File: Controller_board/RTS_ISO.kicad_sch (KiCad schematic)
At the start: 18 parts, among them U7 ADuM1400xRW SOIC-16W, U8 ADuM1400xRW SOIC-16W, U9 ADuM1400xRW SOIC-16W

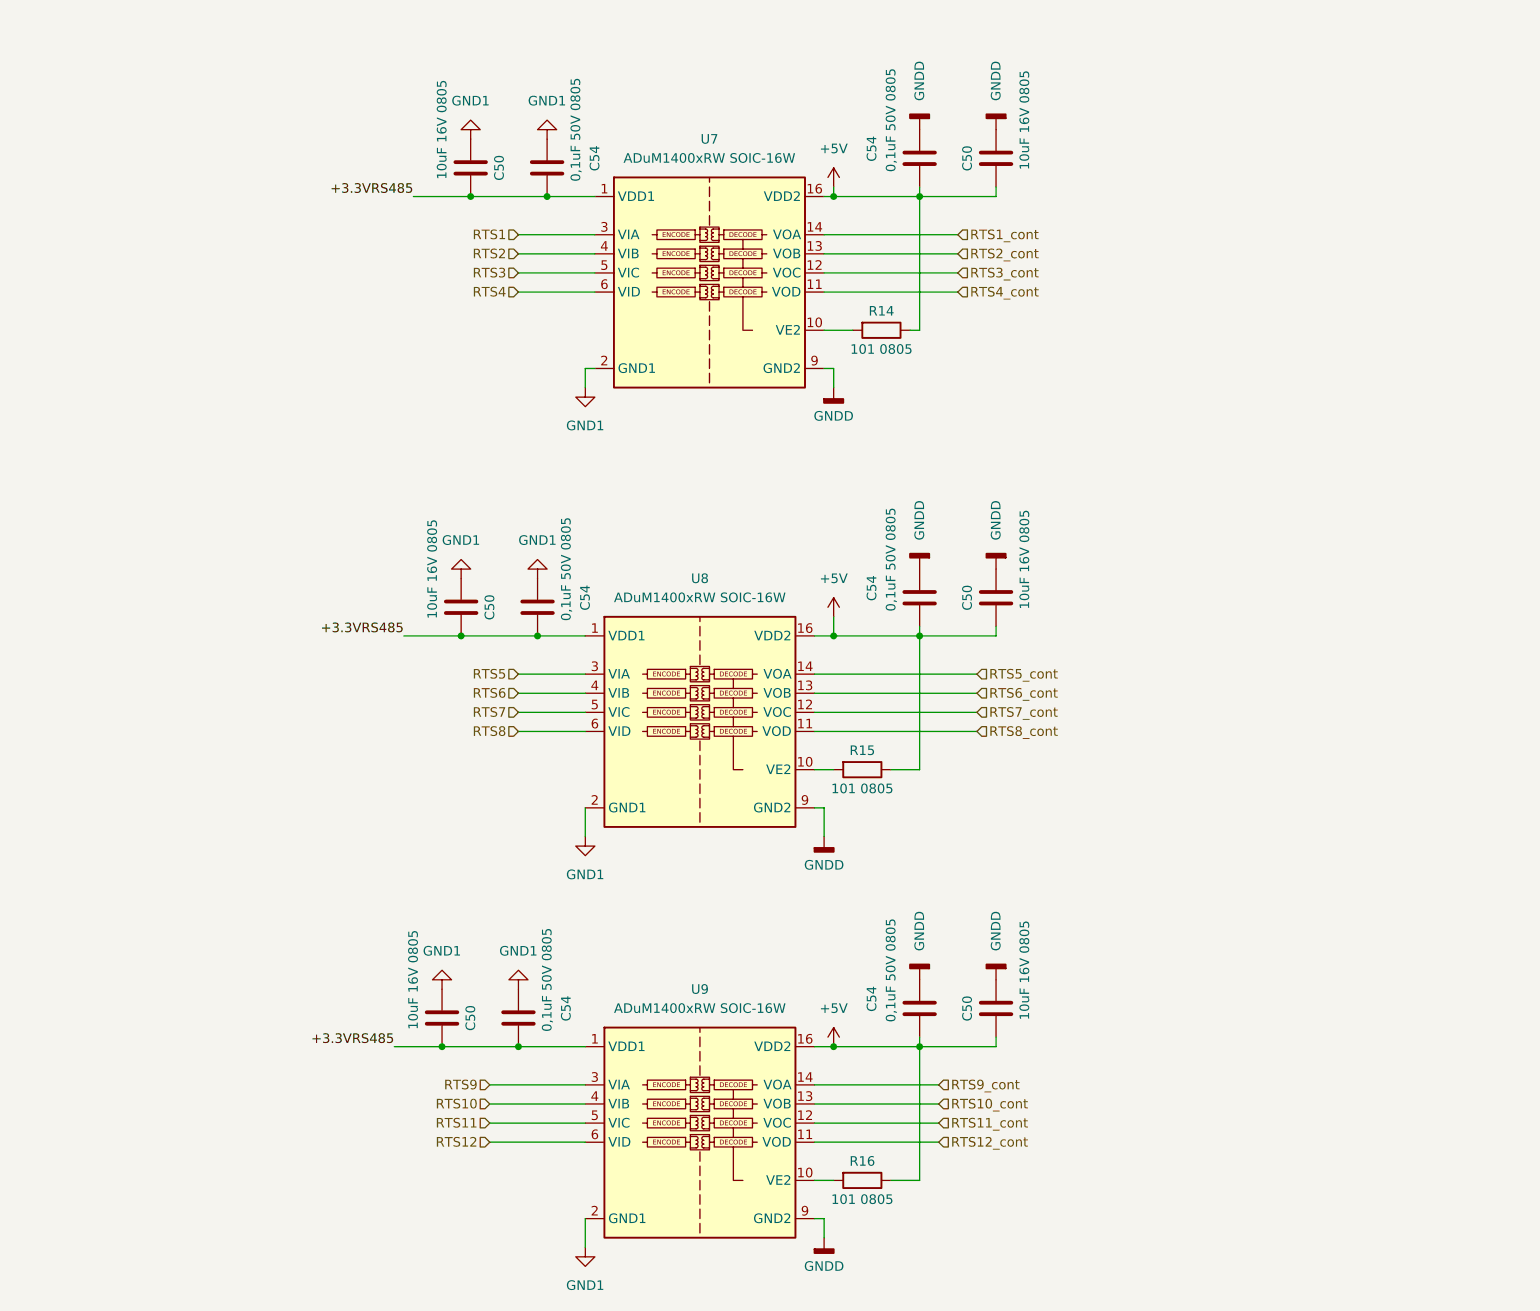
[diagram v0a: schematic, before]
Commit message: Modify MainController Schems and PCB1
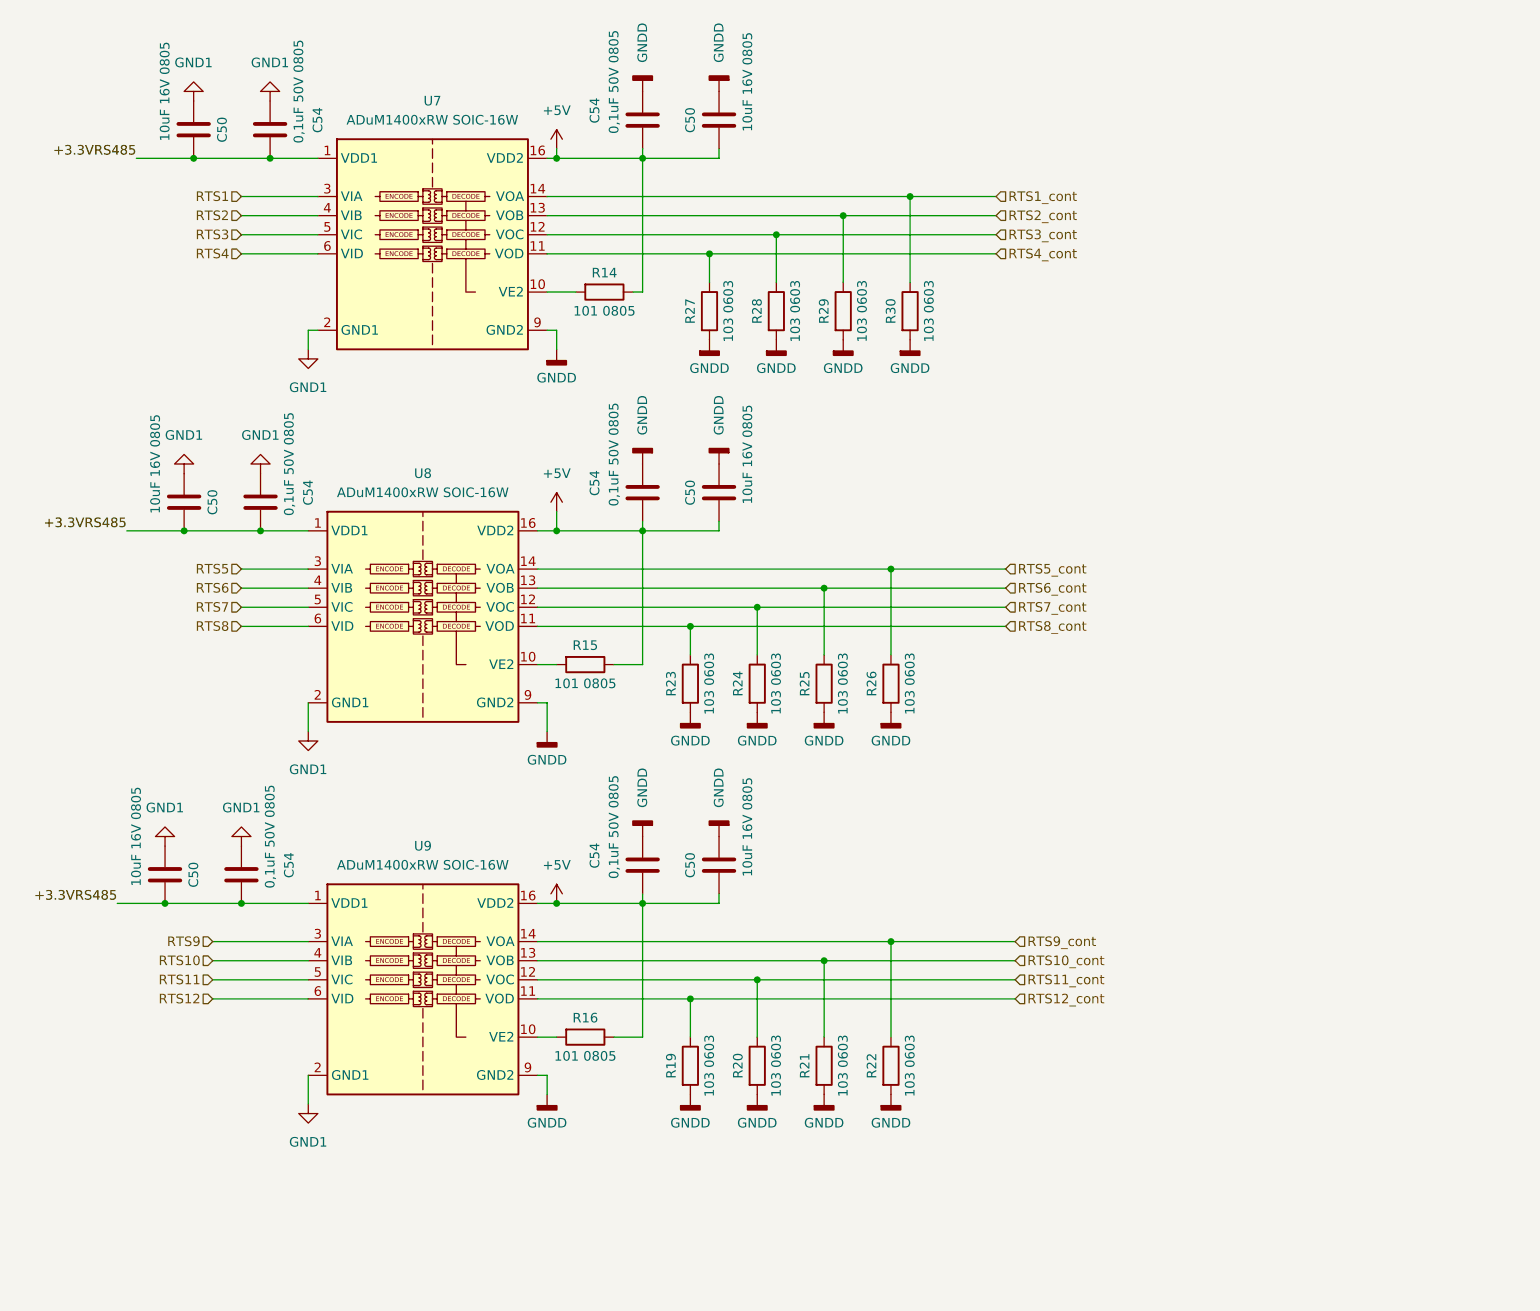
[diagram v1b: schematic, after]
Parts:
- added R19, R20, R21, R22, R23, R24, R25, R26, R27, R28, R29, R30: 103 0603, PCM_4ms_Resistor:R_0603, symbol Device:R
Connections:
- net GNDD: now also R19.2, R20.2, R21.2, R22.2, R23.2, R24.2, R25.2, R26.2, R27.2, R28.2, R29.2, R30.2
- net RTS10_cont: now also R21.1
- net RTS11_cont: now also R20.1
- net RTS12_cont: now also R19.1
- net RTS1_cont: now also R30.1
- net RTS2_cont: now also R29.1
- net RTS3_cont: now also R28.1
- net RTS4_cont: now also R27.1
- net RTS5_cont: now also R26.1
- net RTS6_cont: now also R25.1
- net RTS7_cont: now also R24.1
- net RTS8_cont: now also R23.1
- net RTS9_cont: now also R22.1
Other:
- moved on the sheet: C50, C54, R14, R15, R16, U7, U8, U9

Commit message: Change ISOLATOR 03.06.24
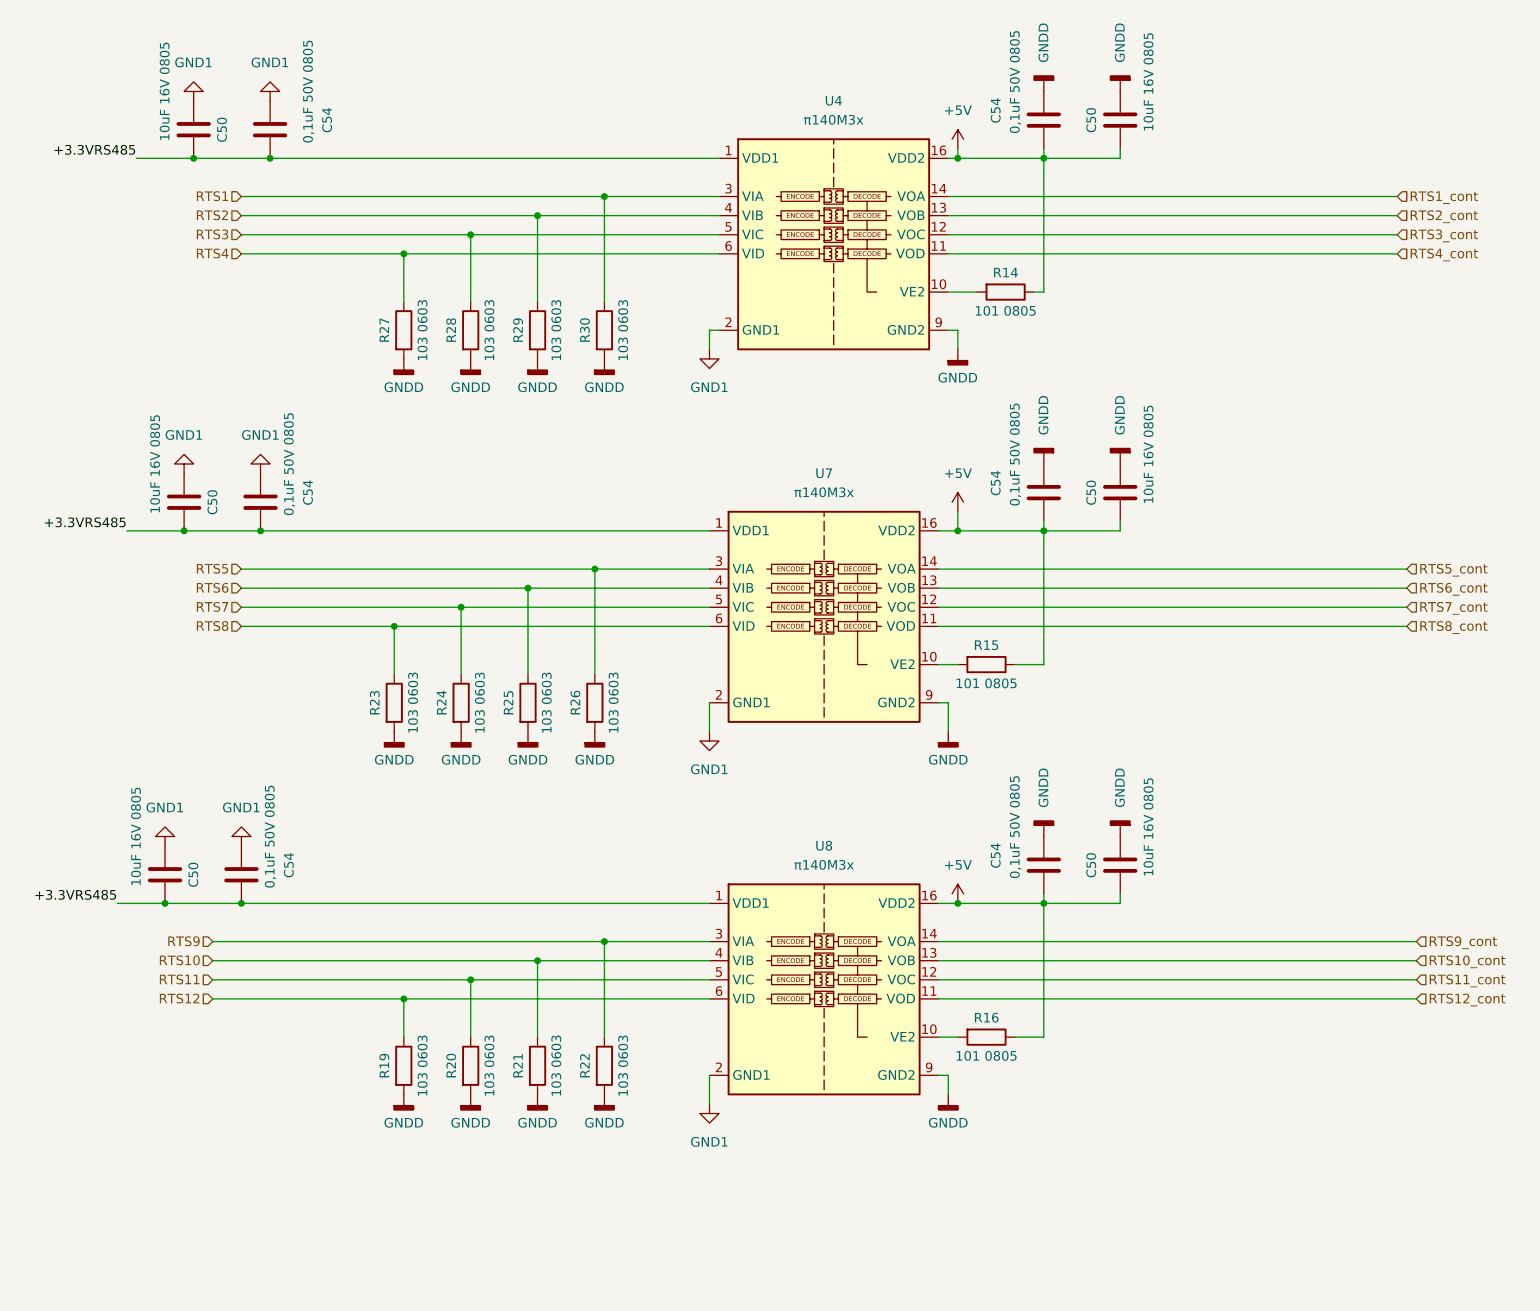
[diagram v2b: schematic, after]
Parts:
- removed U7, U8, U9: ADuM1400xRW SOIC-16W, Package_SO:SOIC-16W_7.5x10.3mm_P1.27mm, symbol Isolator:ADuM1400xRW
- added U4, U7, U8: π140M3x, Package_SO:SOIC-16_3.9x9.9mm_P1.27mm, symbol Isolator:π140M3x
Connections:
- net +3.3VRS485: now also U4.1 (VDD1), U7.1 (VDD1), U8.1 (VDD1)
- net +5V: now also U4.16 (VDD2), U7.16 (VDD2), U8.16 (VDD2)
- net GND1: now also U4.2 (GND1), U4.8 (GND1), U7.2 (GND1), U7.8 (GND1), U8.2 (GND1), U8.8 (GND1)
- net GNDD: now also U4.15 (GND2), U4.9 (GND2), U7.15 (GND2), U7.9 (GND2), U8.15 (GND2), U8.9 (GND2)
- net RTS1: now also R30.1, U4.3 (VIA)
- net RTS10: now also R21.1, U8.4 (VIB)
- net RTS10_cont: now also U8.13 (VOB); no longer R21.1
- net RTS11: now also R20.1, U8.5 (VIC)
- net RTS11_cont: now also U8.12 (VOC); no longer R20.1
- net RTS12: now also R19.1, U8.6 (VID)
- net RTS12_cont: now also U8.11 (VOD); no longer R19.1
- net RTS1_cont: now also U4.14 (VOA); no longer R30.1
- net RTS2: now also R29.1, U4.4 (VIB)
- net RTS2_cont: now also U4.13 (VOB); no longer R29.1
- net RTS3: now also R28.1, U4.5 (VIC)
- net RTS3_cont: now also U4.12 (VOC); no longer R28.1
- net RTS4: now also R27.1, U4.6 (VID)
- net RTS4_cont: now also U4.11 (VOD); no longer R27.1
- net RTS5: now also R26.1, U7.3 (VIA)
- net RTS5_cont: now also U7.14 (VOA); no longer R26.1
- net RTS6: now also R25.1, U7.4 (VIB)
- net RTS6_cont: now also U7.13 (VOB); no longer R25.1
- net RTS7: now also R24.1, U7.5 (VIC)
- net RTS7_cont: now also U7.12 (VOC); no longer R24.1
- net RTS8: now also R23.1, U7.6 (VID)
- net RTS8_cont: now also U7.11 (VOD); no longer R23.1
- net RTS9: now also R22.1, U8.3 (VIA)
- net RTS9_cont: now also U8.14 (VOA); no longer R22.1
- net at R16.2: now also U8.10 (VE2)
- net at R15.2: now also U7.10 (VE2)
- net at R14.2: now also U4.10 (VE2)
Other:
- moved on the sheet: C50, C54, R14, R15, R16, R19, R20, R21, R22, R23, R24, R25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
